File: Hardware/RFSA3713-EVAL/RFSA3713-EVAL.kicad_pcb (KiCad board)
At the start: 2 copper layers, 54.5 x 45.5 mm, 17 parts, among them J1 Conn_Coaxial, J2 Conn_Coaxial, J4 Conn_Coaxial, J5 Conn_Coaxial, J6 Conn_02x05_Odd_Even, SW1 SW_SPDT, SW2 SW_SPDT, SW3 SW_SPDT

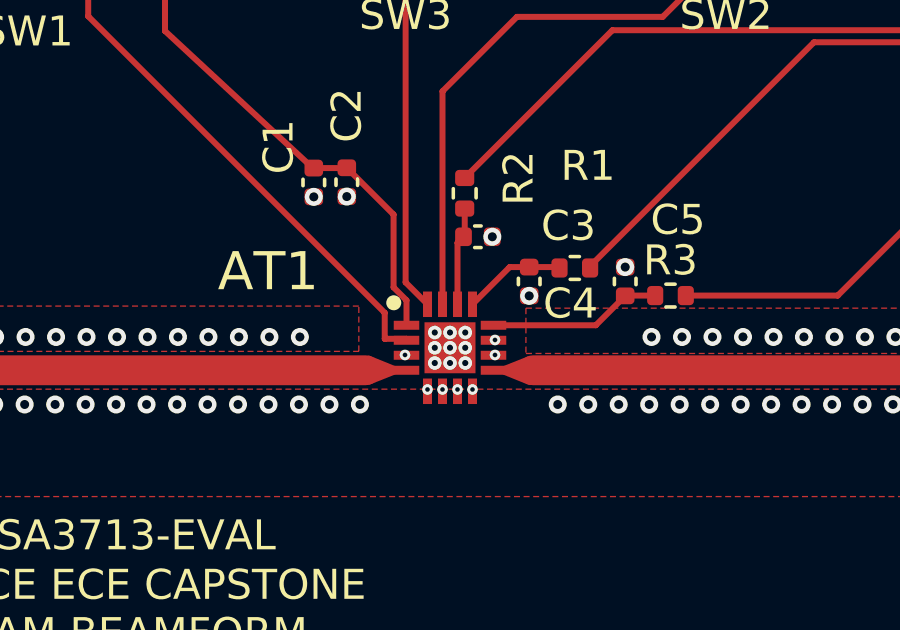
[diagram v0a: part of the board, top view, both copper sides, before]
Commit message: Fixed JLCPCB Errors
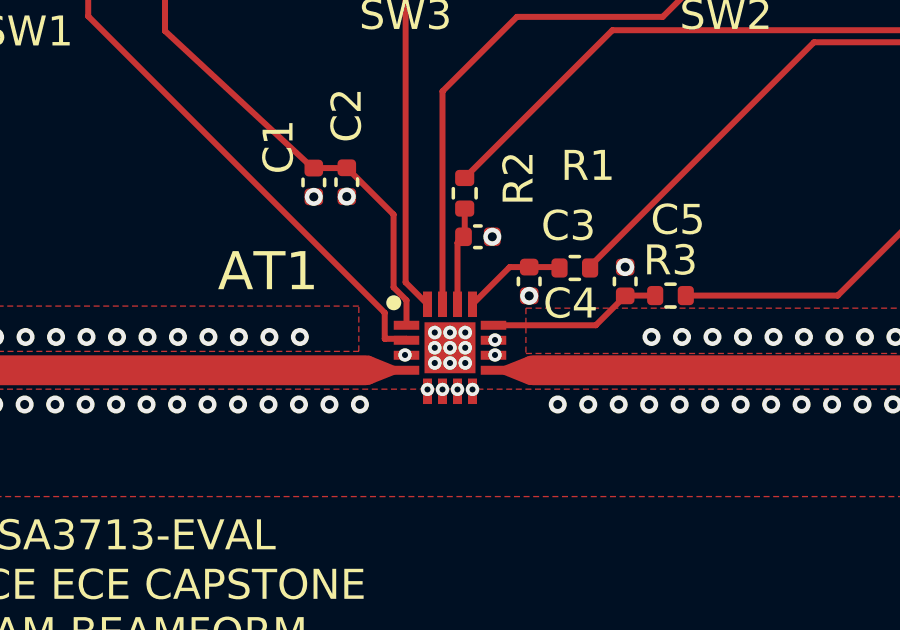
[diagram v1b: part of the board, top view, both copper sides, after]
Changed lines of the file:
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@@
 			(plot_on_all_layers_selection 0x00000000_00000000_00000000_00000000)
 			(disableapertmacros no)
-			(usegerberextensions no)
+			(usegerberextensions yes)
 			(usegerberattributes yes)
 			(usegerberadvancedattributes yes)
@@
 			(sketchdnponfab yes)
 			(crossoutdnponfab yes)
-			(subtractmaskfromsilk no)
+			(subtractmaskfromsilk yes)
 			(outputformat 1)
 			(mirror no)
-			(drillshape 1)
+			(drillshape 0)
 			(scaleselection 1)
-			(outputdirectory "")
+			(outputdirectory "NoCutTest/")
 		)
 	)
@@
 	(via
 		(at 197.55 62.55)
-		(size 0.3556)
-		(drill 0.1524)
+		(size 0.45)
+		(drill 0.2)
 		(layers "F.Cu" "B.Cu")
 		(teardrops
@@
 	(via
 		(at 198.55 62.55)
-		(size 0.3556)
-		(drill 0.1524)
+		(size 0.45)
+		(drill 0.2)
 		(layers "F.Cu" "B.Cu")
 		(teardrops
@@
 	(via
 		(at 199.8 61.4)
-		(size 0.3556)
-		(drill 0.1524)
+		(size 0.45)
+		(drill 0.2)
 		(layers "F.Cu" "B.Cu")
 		(teardrops
@@
 	(via
 		(at 196.8 61.4)
-		(size 0.3556)
-		(drill 0.1524)
+		(size 0.45)
+		(drill 0.2)
 		(layers "F.Cu" "B.Cu")
 		(teardrops
@@
 	(via
 		(at 198.05 62.55)
-		(size 0.3556)
-		(drill 0.1524)
+		(size 0.45)
+		(drill 0.2)
 		(layers "F.Cu" "B.Cu")
 		(teardrops
@@
 	(via
 		(at 199.05 62.55)
-		(size 0.3556)
-		(drill 0.1524)
+		(size 0.45)
+		(drill 0.2)
 		(layers "F.Cu" "B.Cu")
 		(teardrops
@@
 	(via
 		(at 199.8 60.9)
-		(size 0.3556)
-		(drill 0.1524)
+		(size 0.45)
+		(drill 0.2)
 		(layers "F.Cu" "B.Cu")
 		(teardrops
@@
 	)
 	(segment
-		(start 198.75 57.46)
-		(end 198.55 57.66)
+		(start 198.79 56.52)
+		(end 198.79 57.42)
 		(width 0.2)
 		(layer "F.Cu")
@@
 	)
 	(segment
-		(start 198.79 56.52)
-		(end 198.79 57.42)
+		(start 198.55 59.71)
+		(end 198.55 57.66)
 		(width 0.2)
 		(layer "F.Cu")
@@
 	(segment
 		(start 198.55 57.66)
-		(end 198.55 59.71)
+		(end 198.75 57.46)
 		(width 0.2)
 		(layer "F.Cu")
